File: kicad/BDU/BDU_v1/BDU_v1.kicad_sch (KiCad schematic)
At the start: 15 parts, among them J1 pre_aux, J2 high_aux, J3 low_aux, J4 aux 12v, J5 Conn_01x02, J6 Conn_01x02, J7 Conn_01x02, K1 Relay_DPST-NO, K2 Relay_DPST-NO, K3 Relay_DPST-NO, U1 LTV-847S, U2 TRA3-1212

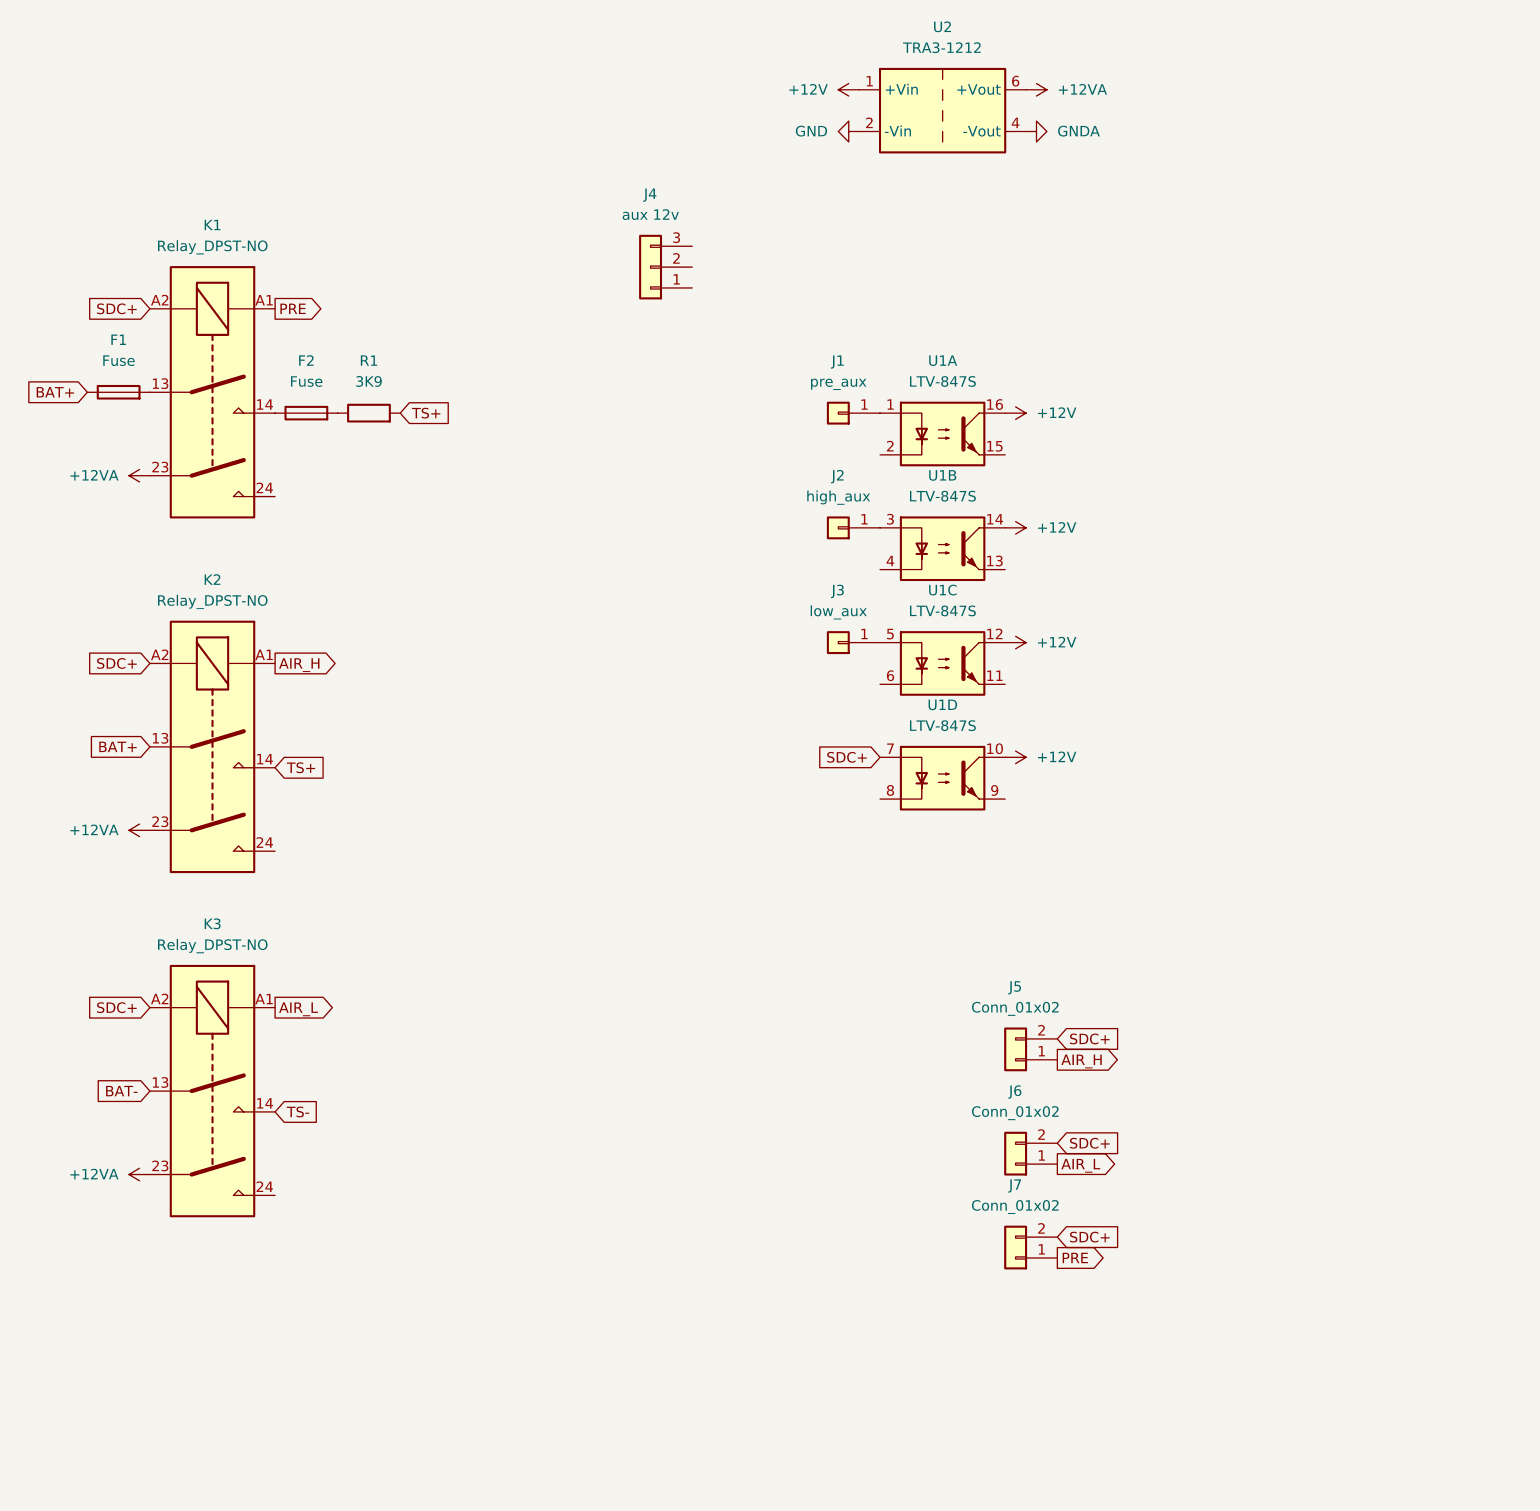
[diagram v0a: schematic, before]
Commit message: bdu
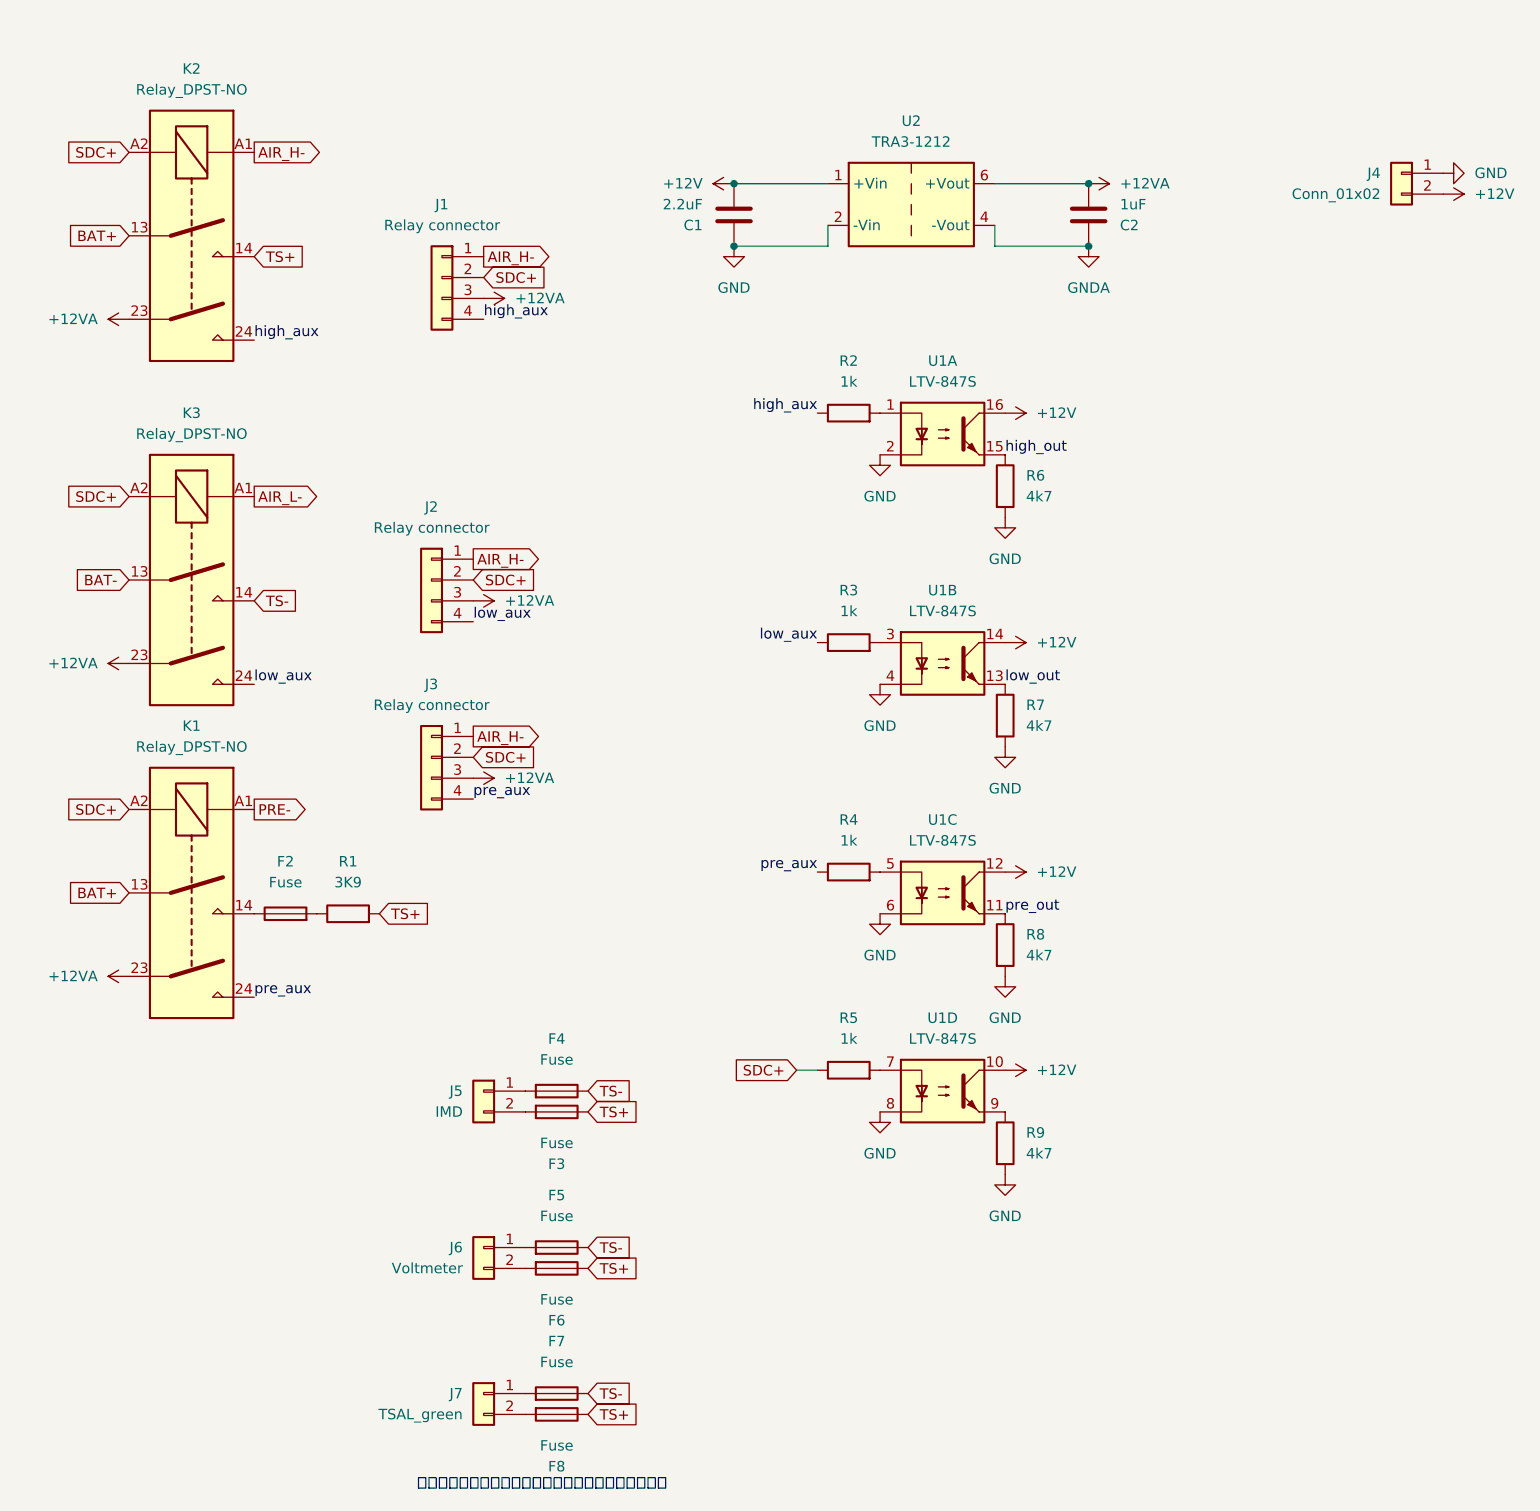
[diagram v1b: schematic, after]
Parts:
- removed F1: Fuse, symbol Device:Fuse
- removed J1: pre_aux, symbol Connector_Generic:Conn_01x01
- removed J2: high_aux, symbol Connector_Generic:Conn_01x01
- removed J3: low_aux, symbol Connector_Generic:Conn_01x01
- removed J4: aux 12v, symbol Connector_Generic:Conn_01x03
- added C1: 2.2uF, symbol Device:C
- added C2: 1uF, symbol Device:C
- added F3, F4, F5, F6, F7, F8: Fuse, symbol Device:Fuse
- added J1, J2, J3: Relay connector, symbol Connector_Generic:Conn_01x04
- added J4: Conn_01x02, symbol Connector_Generic:Conn_01x02
- added R2, R3, R4, R5: 1k, symbol Device:R
- added R6, R7, R8, R9: 4k7, symbol Device:R
- J5: value Conn_01x02 -> IMD
- J6: value Conn_01x02 -> Voltmeter
- J7: value Conn_01x02 -> TSAL_green
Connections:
- net +12V: now also C1.2, J4.2 (Pin_2)
- net +12VA: now also C2.2, J1.3 (Pin_3), J2.3 (Pin_3), J3.3 (Pin_3)
- net BAT+: now also K1.13
- net GND: now also U1.2, U1.4, U1.6, U1.8, C1.1, J4.1 (Pin_1), R6.2, R7.2, R8.2, R9.2
- net GNDA: now also C2.1
- net SDC+: now also J1.2 (Pin_2), J2.2 (Pin_2), J3.2 (Pin_2), R5.1; no longer J5.2 (Pin_2), J6.2 (Pin_2), J7.2 (Pin_2), U1.7
- net TS+: now also F3.1, F6.1, F8.1
- net TS-: now also F4.1, F5.1, F7.1
- net at U1.1: now also R2.2
- net high_out: now reaches U1.15
- net high_out: now also R6.1
- net low_aux: now reaches K3.24
- net low_aux: now also J2.4 (Pin_4), R3.1
- net low_out: now reaches U1.13
- net low_out: now also R7.1
- net at U1.3: now also R3.2
- net pre_out: now reaches U1.11
- net pre_out: now also R8.1
- net at U1.5: now also R4.2
- net at U1.9: now also R9.1
- net high_aux: now reaches K2.24
- net high_aux: now also J1.4 (Pin_4), R2.1
- net pre_aux: now reaches K1.24
- net pre_aux: now also J3.4 (Pin_4), R4.1
- net AIR_H: no longer names the net of J5.1 (Pin_1)
- net AIR_H: now also F4.2; no longer K2.A1
- net AIR_L: no longer names the net of J6.1 (Pin_1)
- net AIR_L: now also F5.2; no longer K3.A1
- net PRE: no longer names the net of J7.1 (Pin_1)
- net PRE: now also F7.2; no longer K1.A1
- new net: F6.2, J6.2 (Pin_2)
- new net: F8.2, J7.2 (Pin_2)
- new net: F3.2, J5.2 (Pin_2)
- new net: R5.2, U1.7
- new net AIR_H-: J1.1 (Pin_1), J2.1 (Pin_1), J3.1 (Pin_1), K2.A1
- new net AIR_L-: K3.A1
- new net PRE-: K1.A1
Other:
- note added: "上述电压检测必须在相应的驱动系统的外壳内部进行。"
- moved on the sheet: F2, K1, K2, K3, R1, U1B, U1C, U1D, U2
